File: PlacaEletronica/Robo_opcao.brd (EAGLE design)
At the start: 139.7 x 148 mm, 101 parts, among them IC1 7805DT, IC2 7805DT, J1 F-1X06-SIP-100-40, J2 S2B-PH-K-S(LF)(SN), J3 ZX62-B-5PA, Q1 SMD-TRANSISTORS-NPN-25V-500MW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, Q2 SMD-TRANSISTORS-NPN-25V-500MW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, Q4 SFH_3716, U1 ESP32-WROOM-32D, U2 AMS1117-3.3, U3 INTERFACE-CP2102-GMR(QFN28)QF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

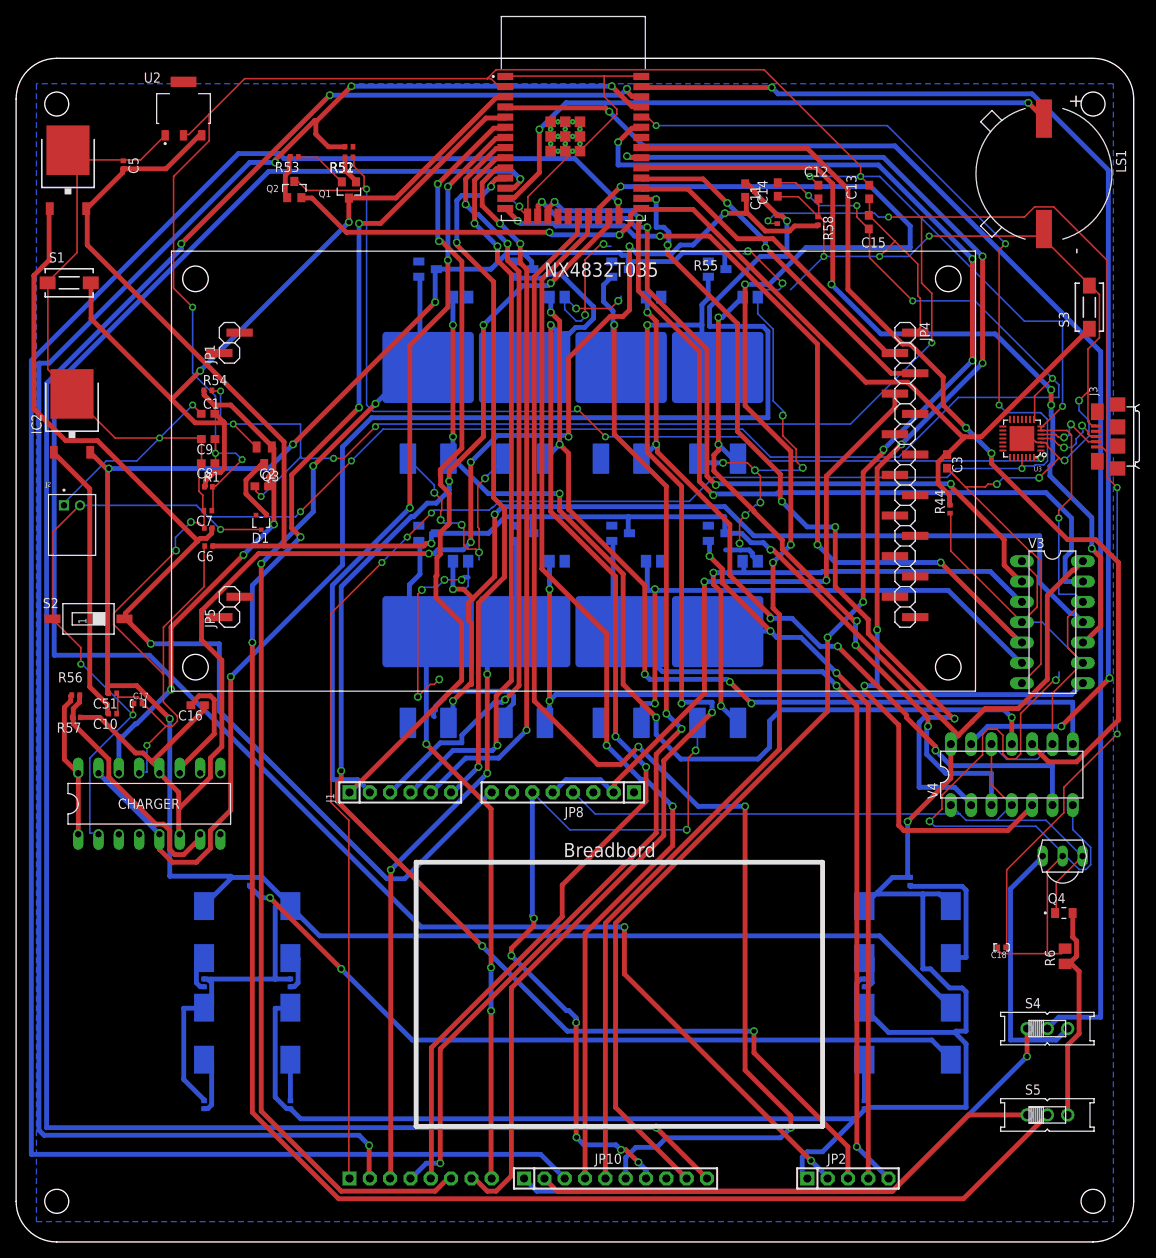
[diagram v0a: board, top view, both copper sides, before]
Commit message: Tudo funcionando perfeitamente antes de implementar upload OTA
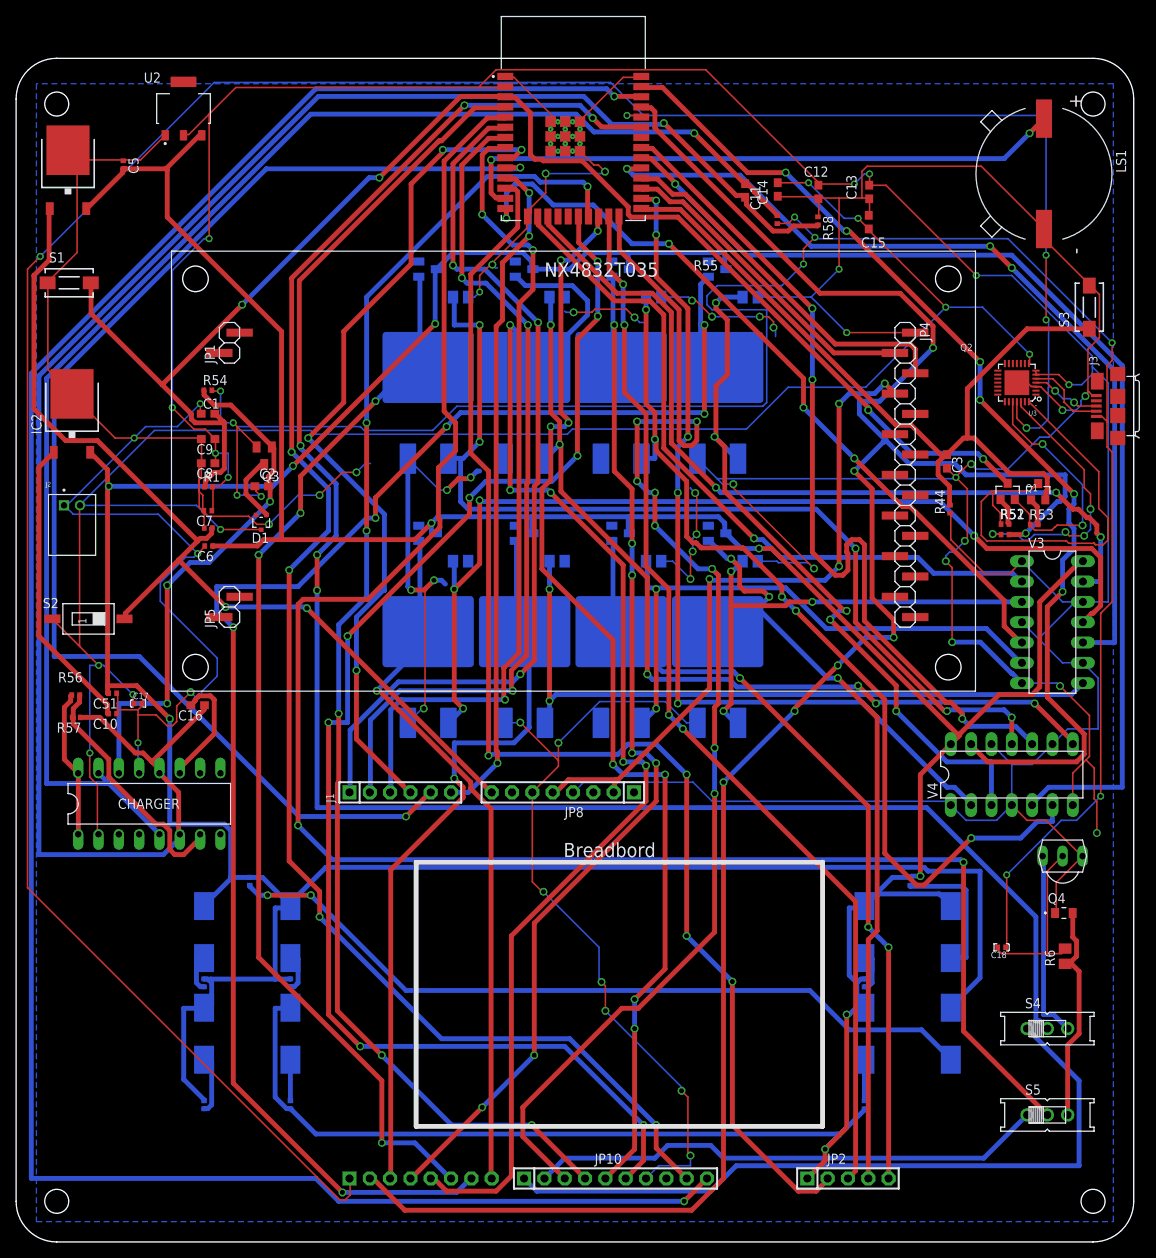
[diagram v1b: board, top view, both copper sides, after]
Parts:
- moved R53 103.3 mm to (127.3, 89.7), turned to 0 degrees
- moved Q2 100.4 mm to (127.8, 93.8)
- moved R51 95.3 mm to (123.6, 88.4), turned to 0 degrees
- moved R52 93.9 mm to (123.6, 89.7), turned to 0 degrees
- moved Q1 90.6 mm to (123.9, 93.8), turned to 0 degrees
- moved U3 7.01 mm to (125.1, 107.4)
- moved J3 3.81 mm to (137.7, 104.5)
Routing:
- net SS: track 255.6 -> 157.5 mm, vias 1 -> 8
- net EN: track 96.8 -> 182.1 mm, vias 2 -> 4
- net DTR: track 129.6 -> 54.9 mm, vias 4 -> 0
- net 5_S: track 89.6 -> 162.2 mm, vias 3 -> 2
- net RX0: track 255.0 -> 324.1 mm, vias 7 -> 5
- net 7_S: track 233.3 -> 164.8 mm, vias 3 -> 4
- net MISO: track 192.7 -> 138.1 mm, vias 4 -> 8
- net B-: track 177.7 -> 230.2 mm, vias 6 -> 1
- net PORT_13~5V: track 149.4 -> 196.0 mm, vias 3 -> 6
- net 8_S: track 177.1 -> 133.5 mm, vias 6 -> 4
- net VP_SENSOR: track 177.5 -> 213.9 mm, vias 1 -> 3
- net MOSI: track 134.4 -> 168.6 mm, vias 2 -> 6
- net N$3: track 0.00 -> 34.1 mm, vias 0 -> 4
- net IO0: track 130.5 -> 101.1 mm, vias 2 -> 0
- net GND_PWM~5V: track 415.1 -> 387.7 mm, vias 3 -> 5
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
